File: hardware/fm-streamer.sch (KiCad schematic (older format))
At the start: 59 parts, among them J1 USB_A, U1 ESP32_DevKit_V1_DOIT, U2 PCM1772PWR, U3 SI4721

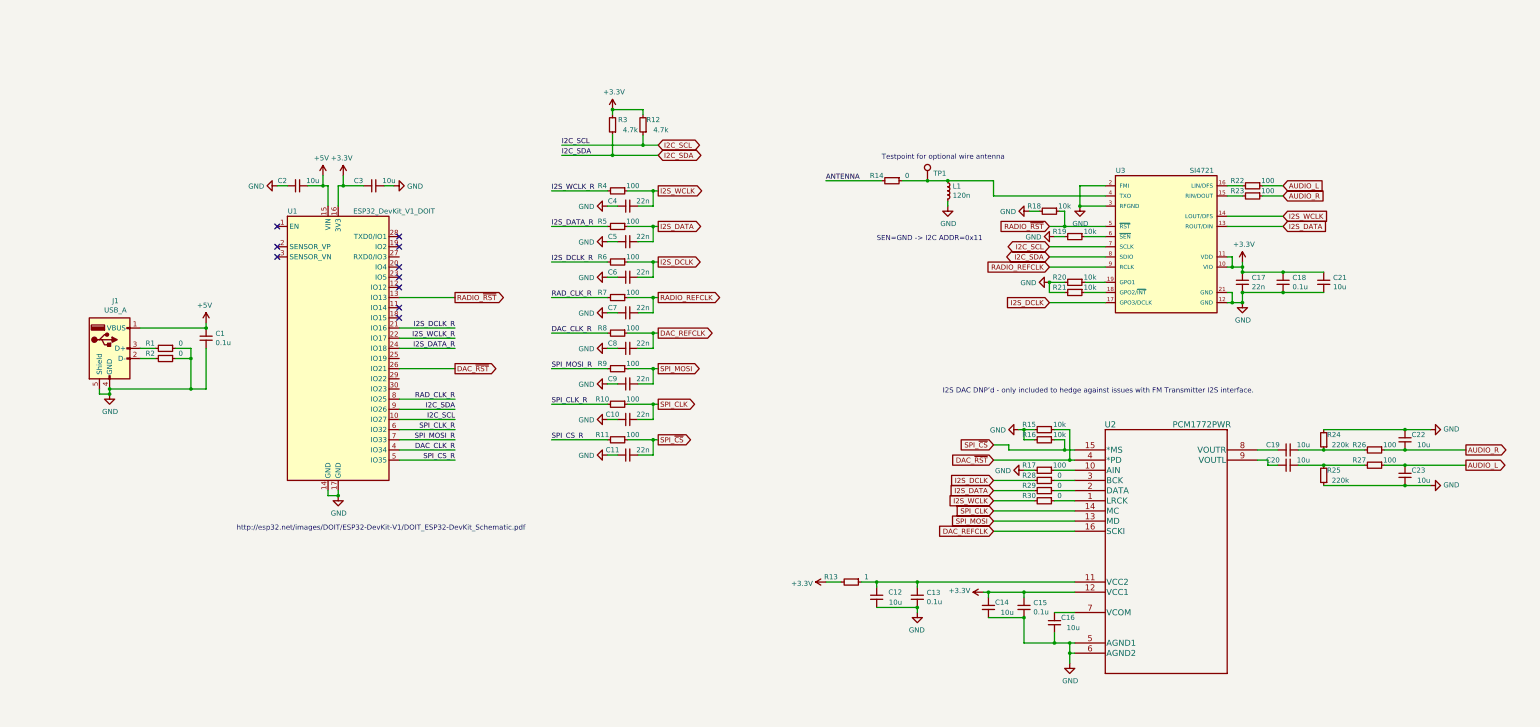
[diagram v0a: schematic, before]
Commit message: Rev0 out to fab
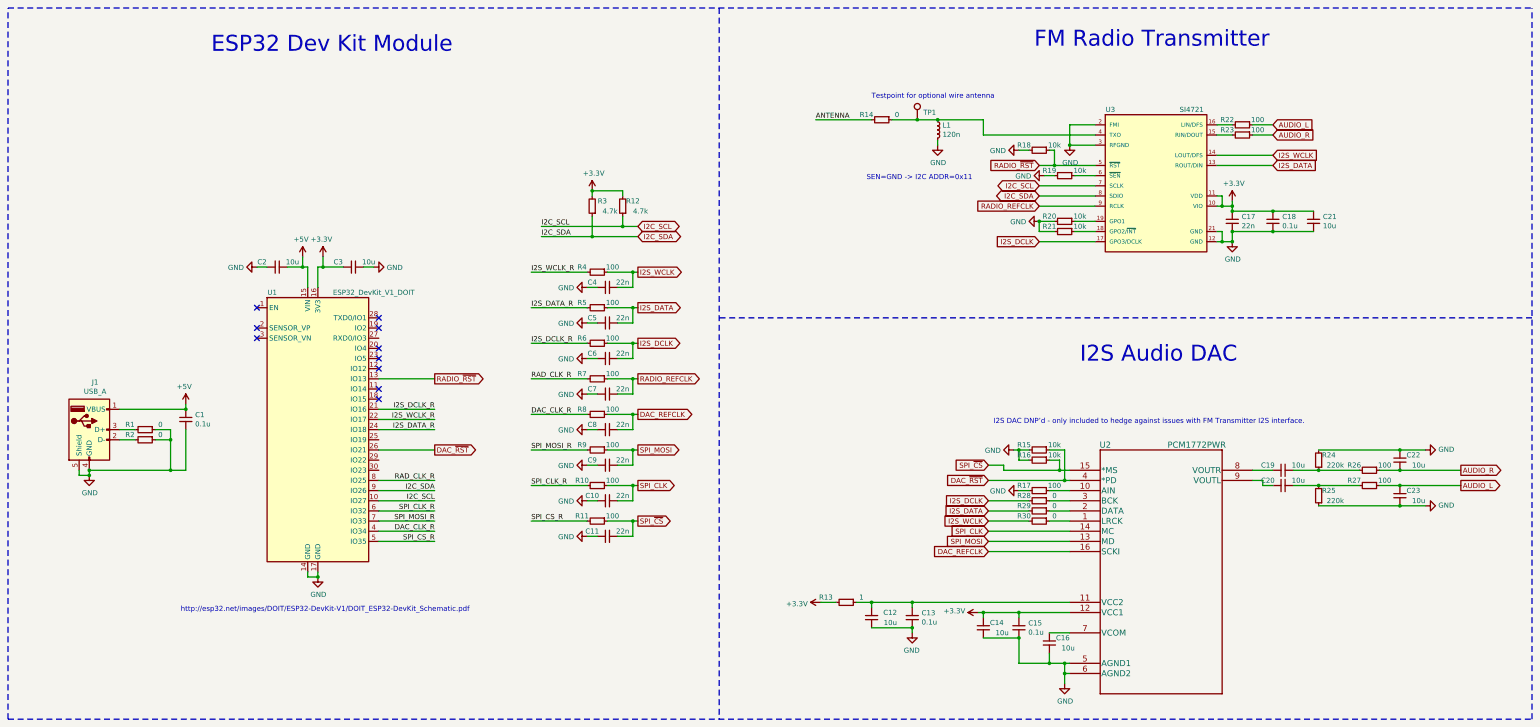
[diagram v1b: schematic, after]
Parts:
- J1: MFG (none) -> Molex; MPN (none) -> 0480371000
- R1, R14, R2, R28, R29, R30: MFG (none) -> Stackpole; MPN (none) -> RMCF0402ZT0R00
- R10, R11, R17, R22, R23, R26, R27, R4, R5, R6, R7, R8, R9: MFG (none) -> Panasonic; MPN (none) -> ERJ-2RKF1000X
- R12, R3: MFG (none) -> Panasonic; MPN (none) -> ERJ-2RKF4701X
- R13: MFG (none) -> Panasonic; MPN (none) -> ERJ-2BQJ1R0X
- R15, R16, R18, R19, R20, R21: MFG (none) -> Panasonic; MPN (none) -> ERJ-2RKF1002X
- R24, R25: MFG (none) -> Panasonic; MPN (none) -> ERJ-2RKF2203X
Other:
- note added: "ESP32 Dev Kit Module"
- note added: "FM Radio Transmitter\n"
- note added: "I2S Audio DAC"
- moved on the sheet: C1, C10, C11, C12, C13, C14, C15, C16, C17, C18, C19, C2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
